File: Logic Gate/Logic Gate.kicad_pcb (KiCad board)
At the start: 2 copper layers, 169.8 x 103 mm, 82 parts, among them J1 Barrel_Jack_MountingPin, J2 Conn_01x02_Socket, Q1 PN2222A, Q10 PN2222A, Q11 PN2222A, Q12 PN2222A, Q13 PN2222A, Q14 PN2222A, Q15 PN2222A, Q16 PN2222A, Q17 PN2222A, Q18 PN2222A, Q2 PN2222A, Q3 PN2222A, Q4 PN2222A, Q5 PN2222A, Q6 PN2222A, Q7 PN2222A, Q8 PN2222A, Q9 PN2222A, SW1 SW_6x6x5, SW10 SW_6x6x5, SW11 SW_6x6x5, SW12 SW_6x6x5, SW13 SW_6x6x5, SW2 SW_6x6x5, SW3 SW_6x6x5, SW4 SW_6x6x5, SW5 SW_6x6x5, SW6 SW_6x6x5, SW7 SW_6x6x5, SW8 SW_6x6x5, SW9 SW_6x6x5, U1 L7805

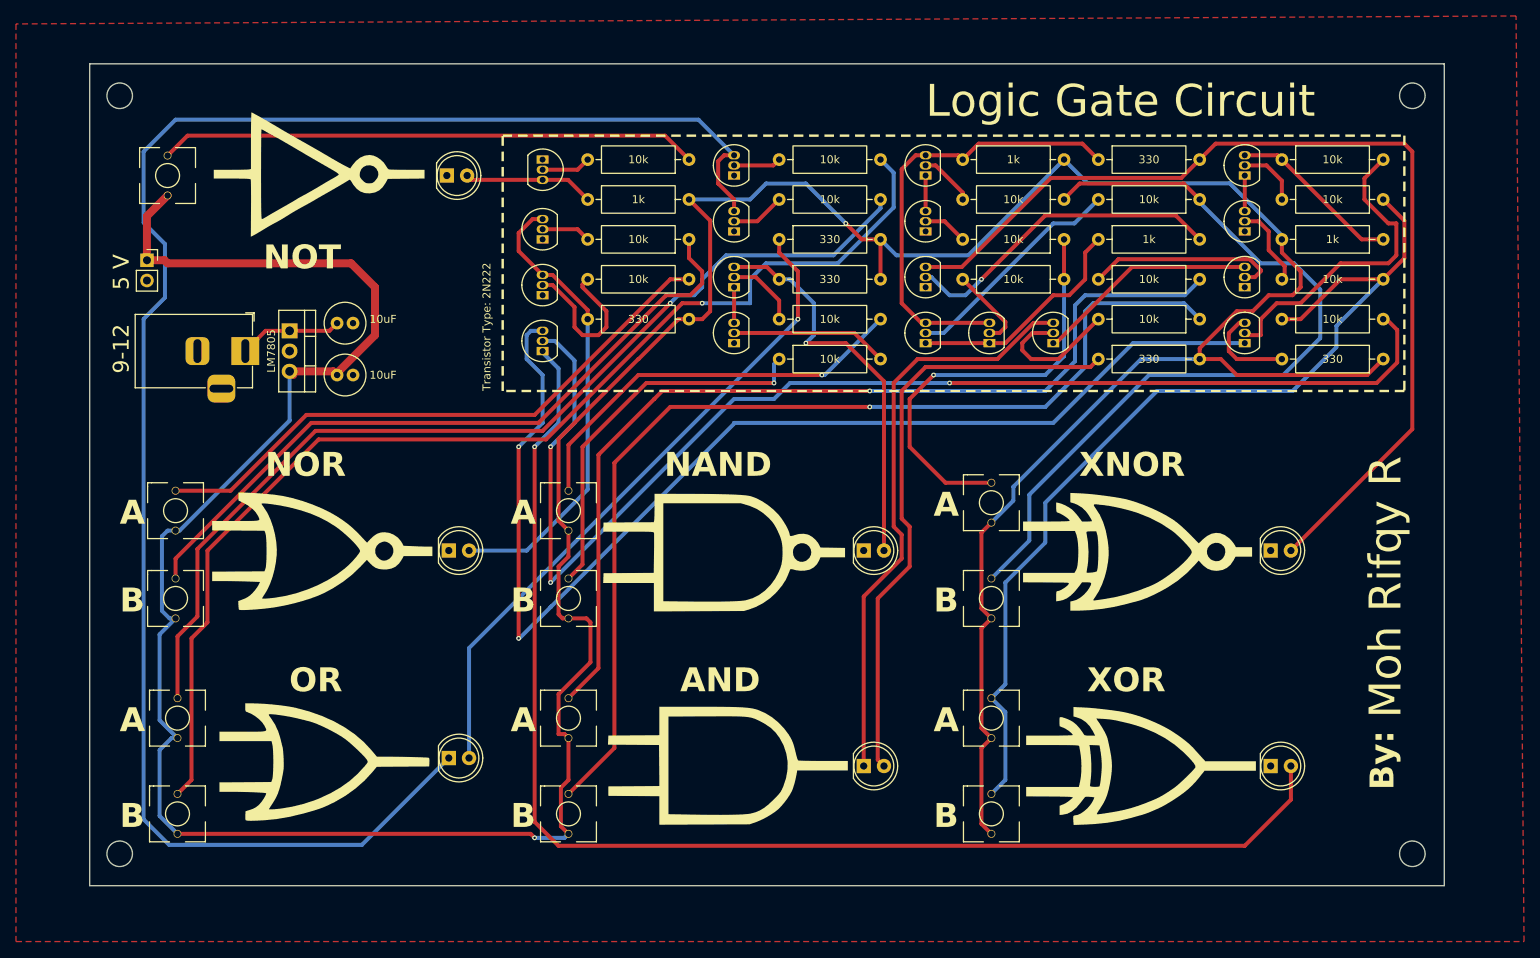
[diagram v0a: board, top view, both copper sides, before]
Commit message: minimum size
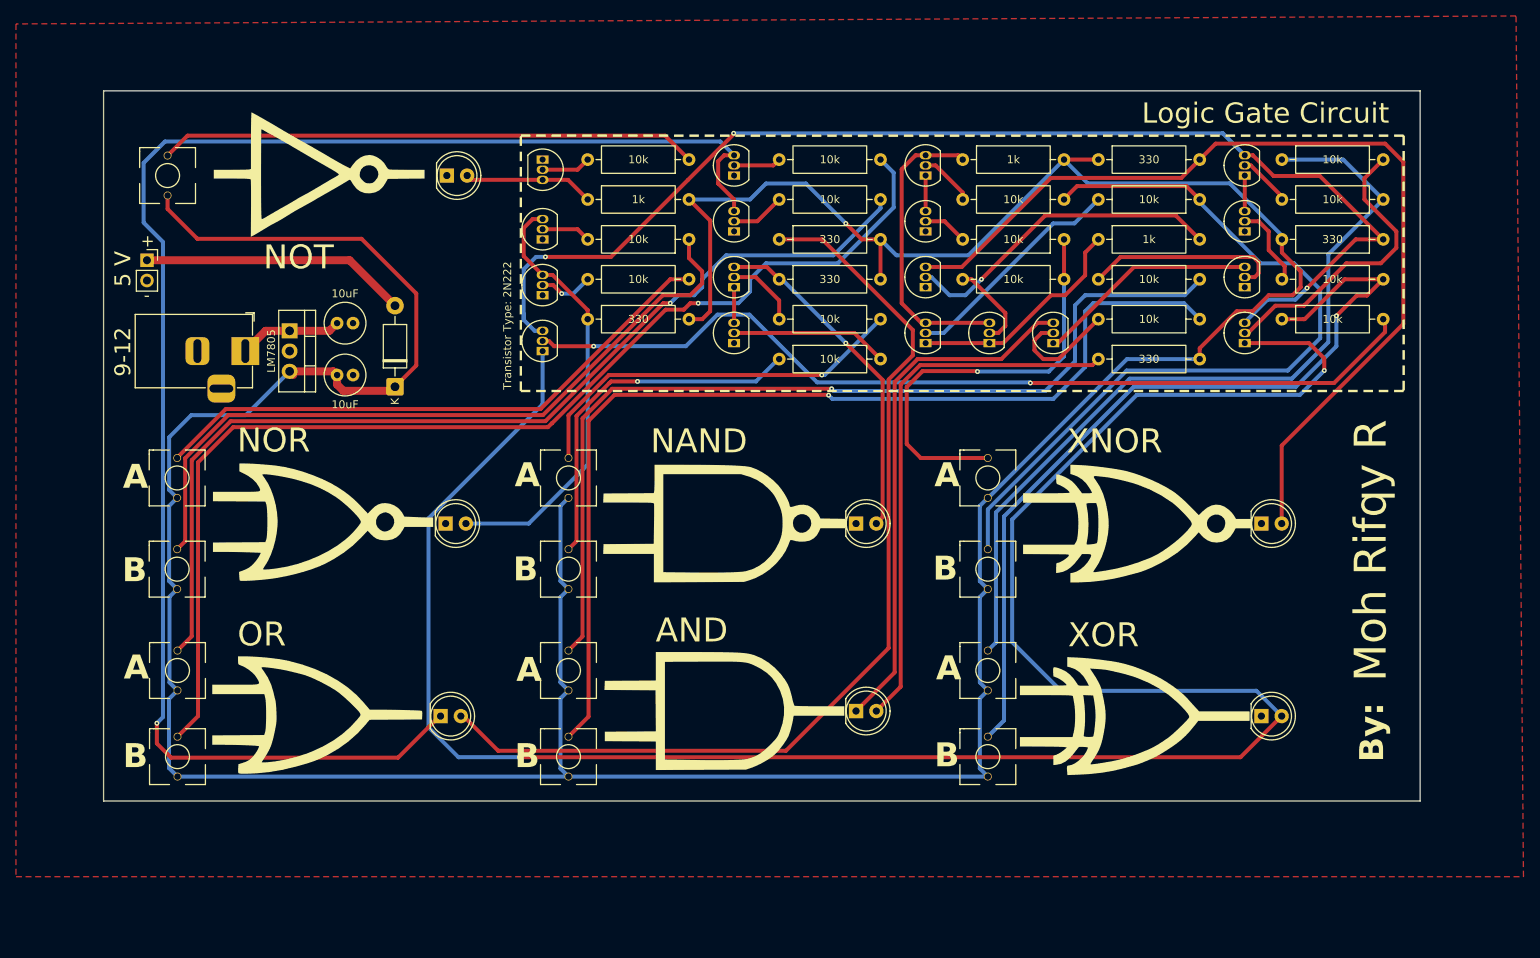
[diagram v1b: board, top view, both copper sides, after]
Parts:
- removed H1, H2, H3, H4: MountingHole, MountingHole:MountingHole_3.2mm_M3
- removed R27: 330, Resistor_THT:R_Axial_DIN0309_L9.0mm_D3.2mm_P12.70mm_Horizontal
- removed the REF** at (150.5, 81.2)
- added D8: 1N4001, Diode_THT:D_DO-41_SOD81_P10.16mm_Horizontal, F.Cu at (103.5, 77.5)
- added REF**: KiCad-Logo2_40mm_SilkScreen, Symbol:KiCad-Logo2_40mm_SilkScreen, B.Cu at (153.7, 74.1)
- R15: value 1k -> 330
- moved SW11 7.19 mm to (177.8, 123.8)
- moved SW2 7.18 mm to (125.2, 123.8)
- moved SW4 7.18 mm to (76.2, 123.8)
- moved D1 6.96 mm to (161.3, 118.1)
- moved G*** 6.87 mm to (145.8, 117.6)
- moved D6 6.36 mm to (212.1, 118.7)
- moved G*** 6.30 mm to (198.5, 118.7)
- moved SW10 5.99 mm to (177.8, 113.0)
- moved SW1 5.97 mm to (125.2, 113.0)
- moved SW3 5.97 mm to (76.2, 113.0)
- moved G*** 5.96 mm to (93.3, 118.1)
- moved D2 5.35 mm to (109.2, 118.7)
- moved SW9 4.10 mm to (76.2, 88.9)
- moved SW6 4.10 mm to (125.2, 88.9)
- moved SW12 3.70 mm to (177.8, 100.3)
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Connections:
- J2 pad 1: +5V -> Net-(D8-A)
- Q12 pad 1: Net-(Q12-E) -> Net-(D6-A)
- Q12 pad 3: Net-(Q12-C) -> Net-(Q10-C)
- Q13 pad 3: Net-(Q12-E) -> Net-(Q10-C)
- R17 pad 1: Net-(R16-Pad1) -> Net-(R17-Pad1)
- R18 pad 1: Net-(Q10-C) -> Net-(R16-Pad1)
- R19 pad 1: Net-(R16-Pad1) -> Net-(R17-Pad1)
- R26 pad 1: Net-(Q14-C) -> +5V
- SW11 pad 1: Net-(R16-Pad1) -> Net-(R17-Pad1)
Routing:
- net Net-(Q12-E): track 148.7 -> 0.00 mm, vias 2 -> 0
- net Net-(Q10-C): track 21.7 -> 152.1 mm, vias 0 -> 3
- net Net-(D6-A): track 163.7 -> 276.2 mm, vias 1 -> 2
- net Net-(R17-Pad1): track 0.00 -> 105.3 mm, vias 0 -> 1
- net Net-(Q13-B): track 158.0 -> 116.2 mm, vias 3 -> 2
- net Net-(D2-A): track 83.0 -> 123.5 mm, vias 1 -> 0
- net Net-(D8-A): track 0.00 -> 33.4 mm
- net Net-(R16-Pad1): track 123.2 -> 103.7 mm
- net Net-(D2-K): track 216.9 -> 197.7 mm, vias 0 -> 1
- net Net-(Q14-C): track 56.1 -> 37.4 mm
- net +5V: track 497.3 -> 480.6 mm, vias 2 -> 1
- net Net-(Q9-B): track 20.0 -> 6.84 mm, vias 0 -> 1
- net Net-(Q12-C): track 11.1 -> 0.00 mm
- net Net-(D4-A): track 50.3 -> 42.8 mm
- net Net-(D1-A): track 75.7 -> 68.3 mm
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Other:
- board size 169.8 x 103 mm -> 165 x 89 mm
- board text added: "+"
- board text added: "-"
